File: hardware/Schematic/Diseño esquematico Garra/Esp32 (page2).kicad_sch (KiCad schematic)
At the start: 2 parts, among them U2 ESP32-WROOM-32

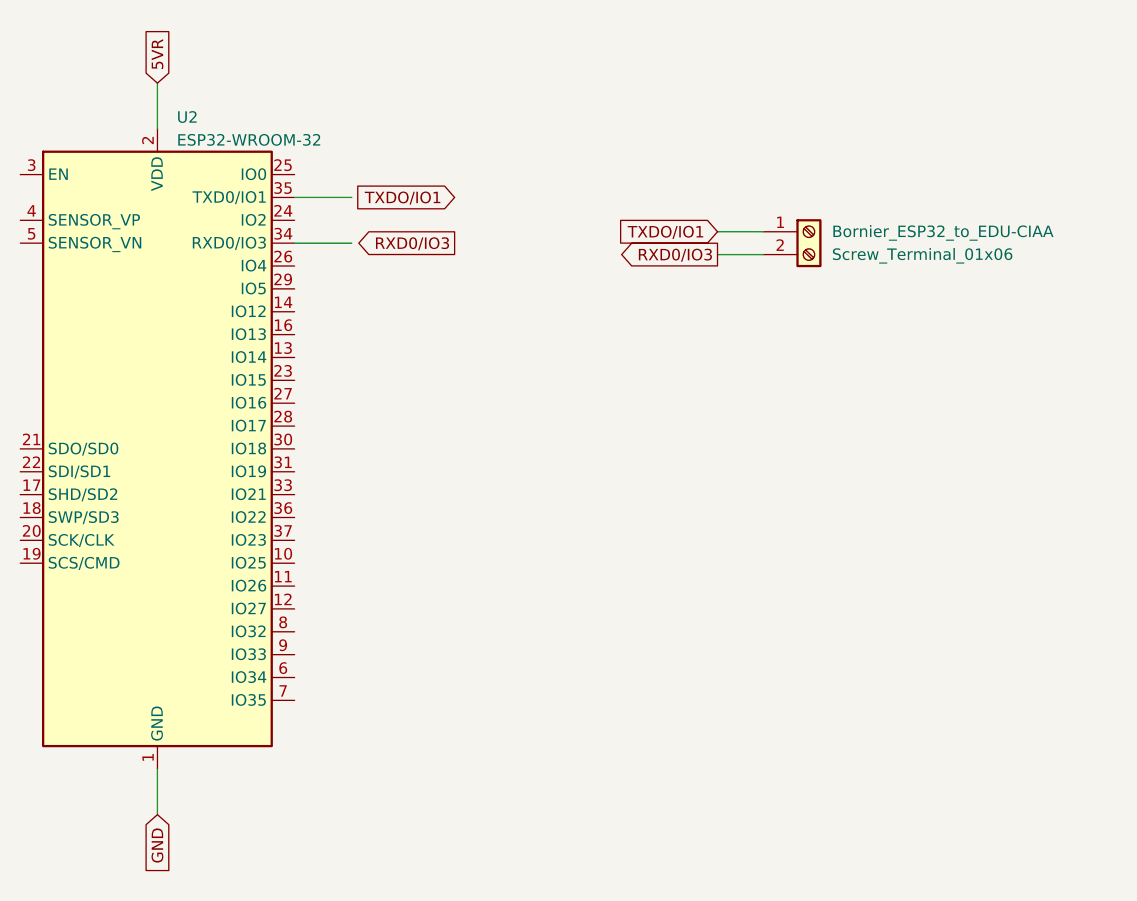
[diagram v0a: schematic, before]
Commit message: Fixes to Schematic
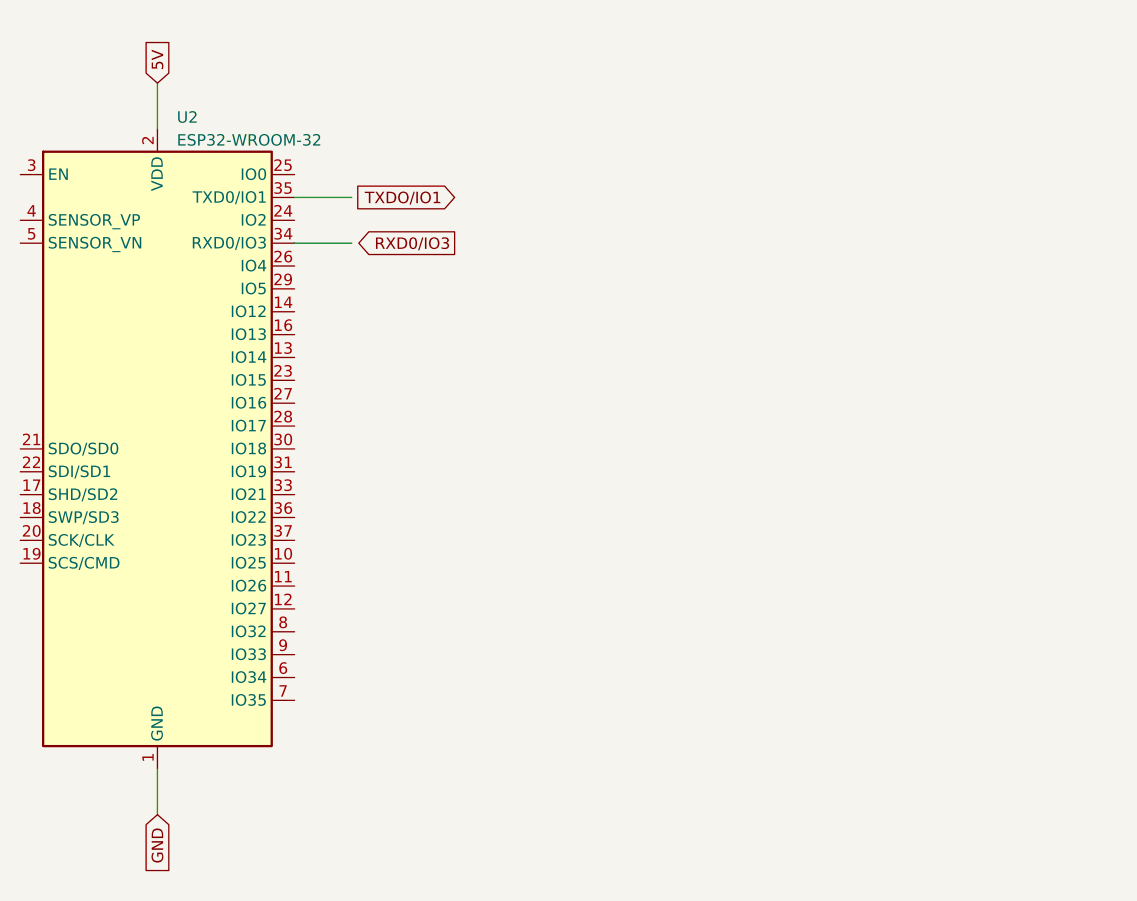
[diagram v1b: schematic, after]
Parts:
- removed Bornier_ESP32_to_EDU-CIAA: Screw_Terminal_01x06, ProyectoTdL:TerminalBlock_bornier-2_P5.08mm, symbol Connector:Screw_Terminal_01x02
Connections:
- net 5VR renamed 5V
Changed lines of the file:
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@@
-	(wire
-		(pts
-			(xy 203.2 69.85) (xy 208.28 69.85)
-		)
-		(stroke
-			(width 0)
-			(type default)
-		)
-	)
 	(wire
 		(pts
 			(xy 140.97 53.34) (xy 140.97 58.42)
-		)
-		(stroke
-			(width 0)
-			(type default)
-		)
-	)
-	(wire
-		(pts
-			(xy 203.2 72.39) (xy 208.28 72.39)
 		)
 		(stroke
@@
 		)
 	)
-	(global_label "RXD0{slash}IO3"
-		(shape output)
-		(at 203.2 72.39 180)
-		(effects
-			(font
-				(size 1.27 1.27)
-			)
-			(justify right)
-		)
-		(property "Intersheetrefs" "${INTERSHEET_REFS}"
-			(at 203.2 72.39 0)
-			(effects
-				(font
-					(size 1.27 1.27)
-				)
-				(hide yes)
-			)
-		)
-	)
-	(global_label "TXDO{slash}IO1"
-		(shape input)
-		(at 203.2 69.85 180)
-		(effects
-			(font
-				(size 1.27 1.27)
-			)
-			(justify right)
-		)
-		(property "Intersheetrefs" "${INTERSHEET_REFS}"
-			(at 203.2 69.85 0)
-			(effects
-				(font
-					(size 1.27 1.27)
-				)
-				(hide yes)
-			)
-		)
-	)
-	(global_label "5VR"
+	(global_label "5V"
 		(shape input)
 		(at 140.97 53.34 90)
@@
 					(unit 1)
 				)
-			)
-		)
-	)
-	(symbol
-		(lib_id "Connector:Screw_Terminal_01x02")
-		(at 213.36 69.85 0)
-		(unit 1)
-		(exclude_from_sim no)
-		(in_bom yes)
-		(on_board yes)
-		(dnp no)
-		(fields_autoplaced yes)
-		(property "Reference" "Bornier_ESP32_to_EDU-CIAA"
-			(at 215.9 69.8499 0)
-			(effects
-				(font
-					(size 1.27 1.27)
-				)
-				(justify left)
-			)
-		)
-		(property "Value" "Screw_Terminal_01x06"
-			(at 215.9 72.3899 0)
-			(effects
-				(font
-					(size 1.27 1.27)
-				)
-				(justify left)
-			)
-		)
-		(property "Footprint" "ProyectoTdL:TerminalBlock_bornier-2_P5.08mm"
-			(at 213.36 69.85 0)
-			(effects
-				(font
-					(size 1.27 1.27)
-				)
-				(hide yes)
-			)
-		)
-		(property "Datasheet" "~"
-			(at 213.36 69.85 0)
-			(effects
-				(font
-					(size 1.27 1.27)
-				)
-				(hide yes)
-			)
-		)
-		(property "Description" "Generic screw terminal, single row, 01x02, script generated (kicad-library-utils/schlib/autogen/connector/)"
-			(at 213.36 69.85 0)
-			(effects
-				(font
-					(size 1.27 1.27)
-				)
-				(hide yes)
-			)
-		)
-		(pin "2"
-		)
-		(pin "1"
-		)
-		(instances
-			(project "Diseño esquematico Garra"
-				(path "/a88248f6-7b70-4a9d-b538-4e8e42a3a066/dc254582-8718-45aa-925a-e29d982f97f0"
-					(reference "Bornier_ESP32_to_EDU-CIAA")
-					(unit 1)
-				)
